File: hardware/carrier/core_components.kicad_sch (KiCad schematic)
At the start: 54 parts, among them J1 PANEL, J2 CARDKB, J3 HAPTIC, J4 EXT_LED, J5 PIEZ, M1 Walter, Q1 UMH3N, Q2 SI1308EDL, Q3 MMST3904, SW1 SKQGAFE010, U1 CP2102N-A02-GQFN24, U2 SN74LVC2G126DCUR, U3 DRV2605LDGSR, U4 LIS2DW12TR

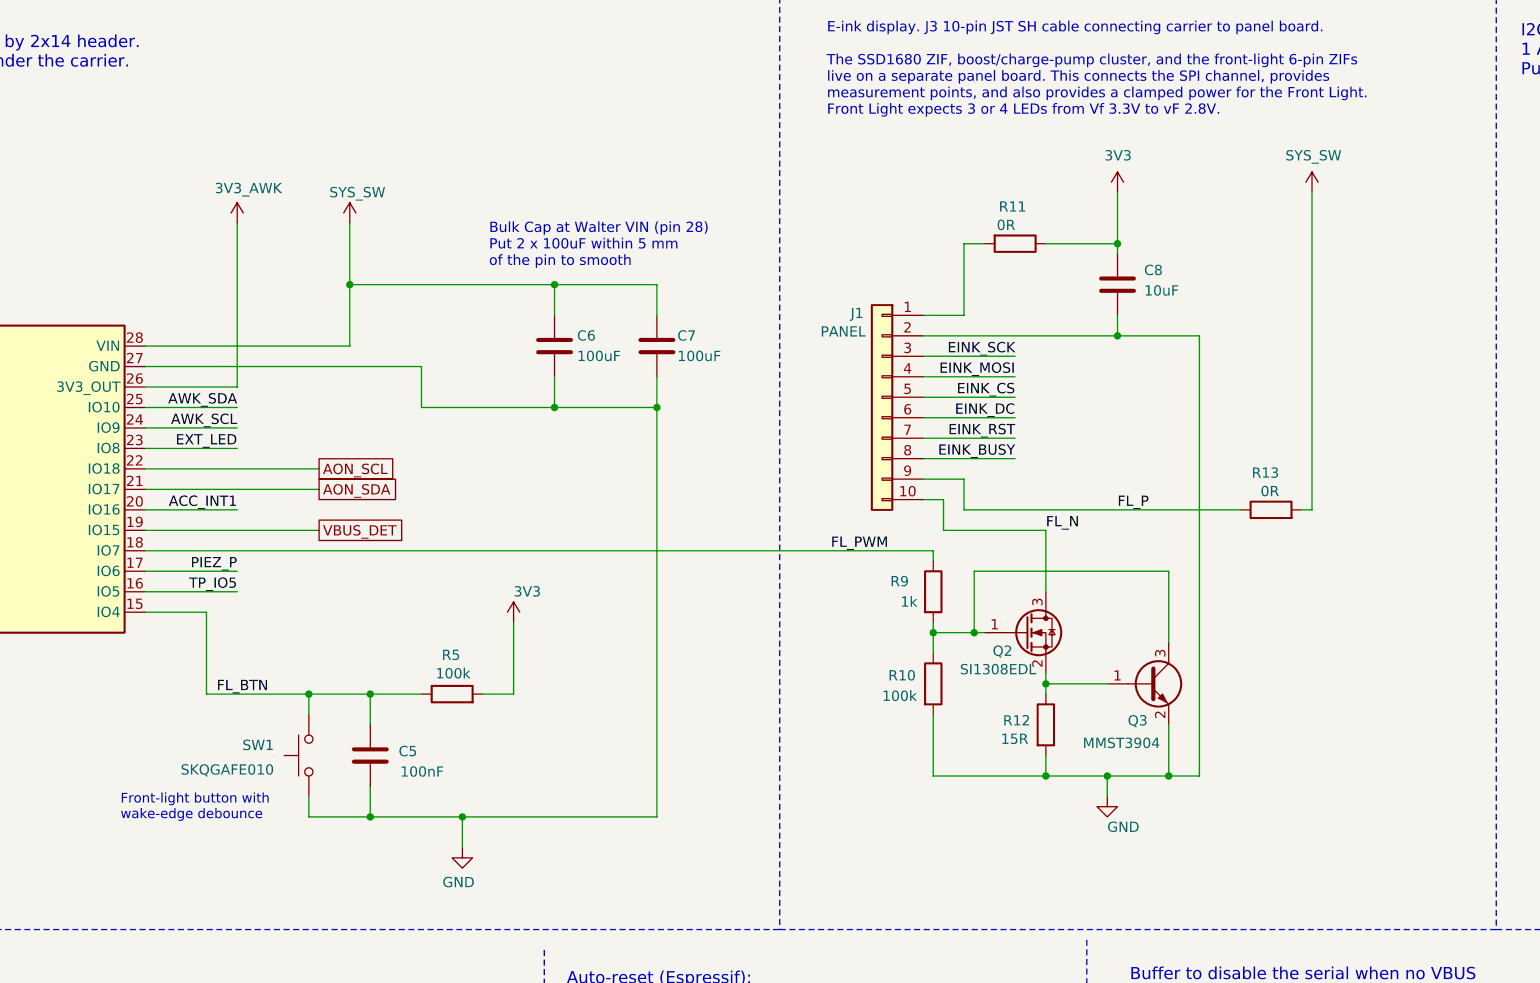
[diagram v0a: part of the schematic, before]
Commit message: Attempt to layout the PCB
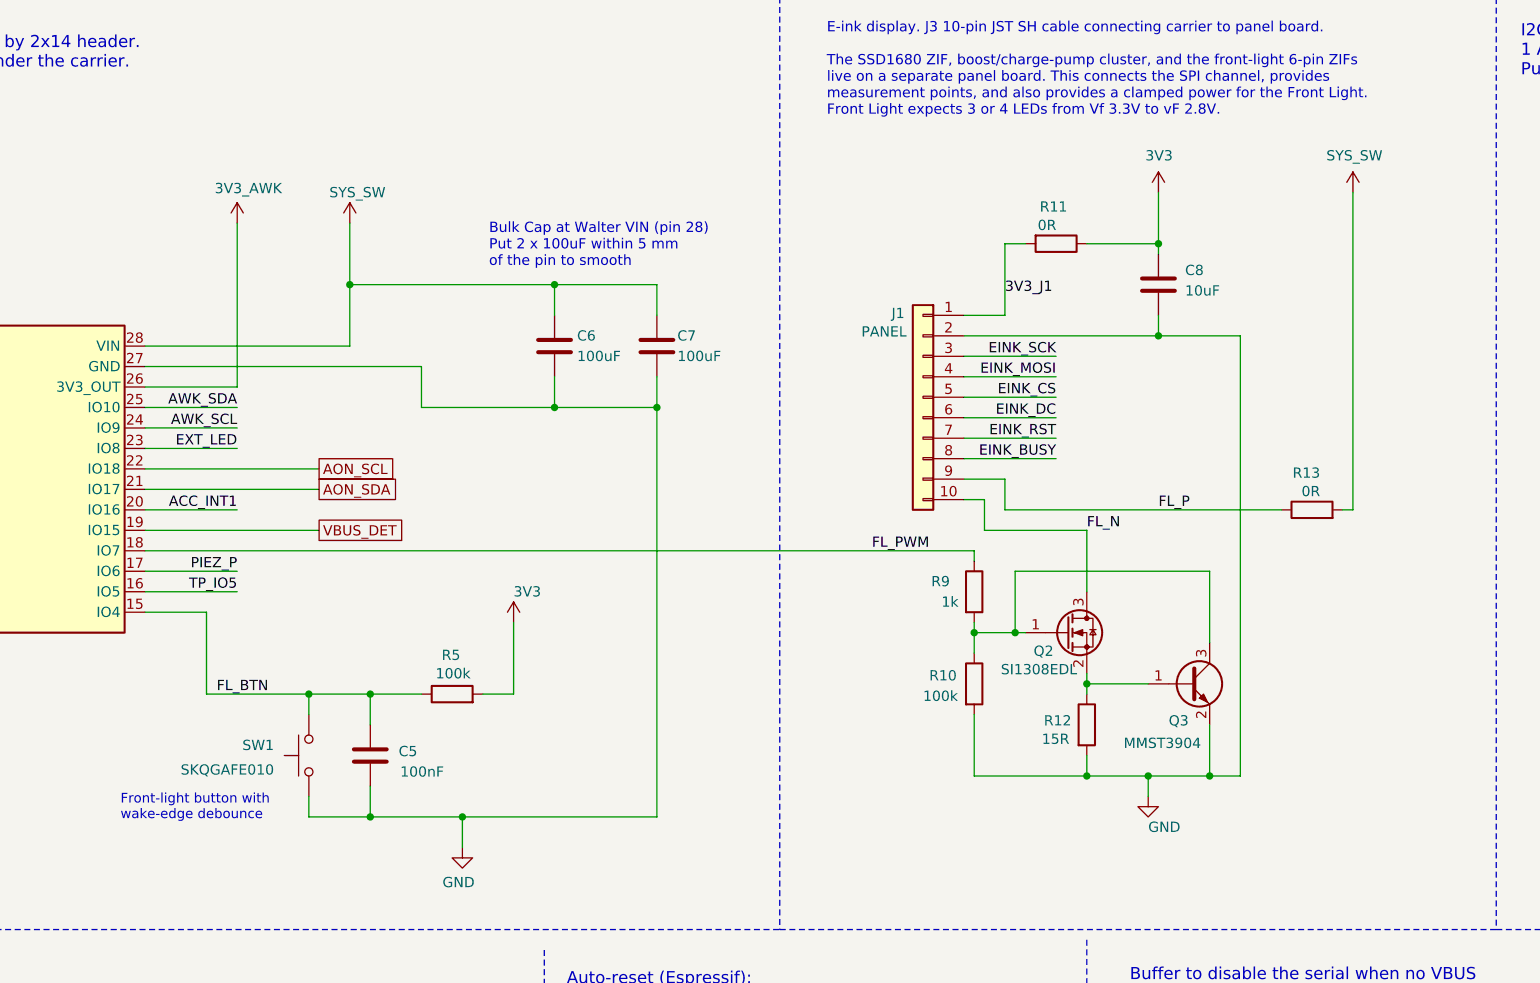
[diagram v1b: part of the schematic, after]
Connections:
- net 3V3_J1: now reaches J1.1 (Pin_1), R11.2
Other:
- moved on the sheet: C8, J1, Q2, Q3, R10, R11, R12, R13, R9
